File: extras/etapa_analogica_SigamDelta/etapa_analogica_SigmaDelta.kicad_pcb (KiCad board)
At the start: 2 copper layers, 63.5 x 78.8 mm, 19 parts, among them P1 CONN_02X10, P2 CONN_01X03, P3 CONN_02X10, P4 BNC

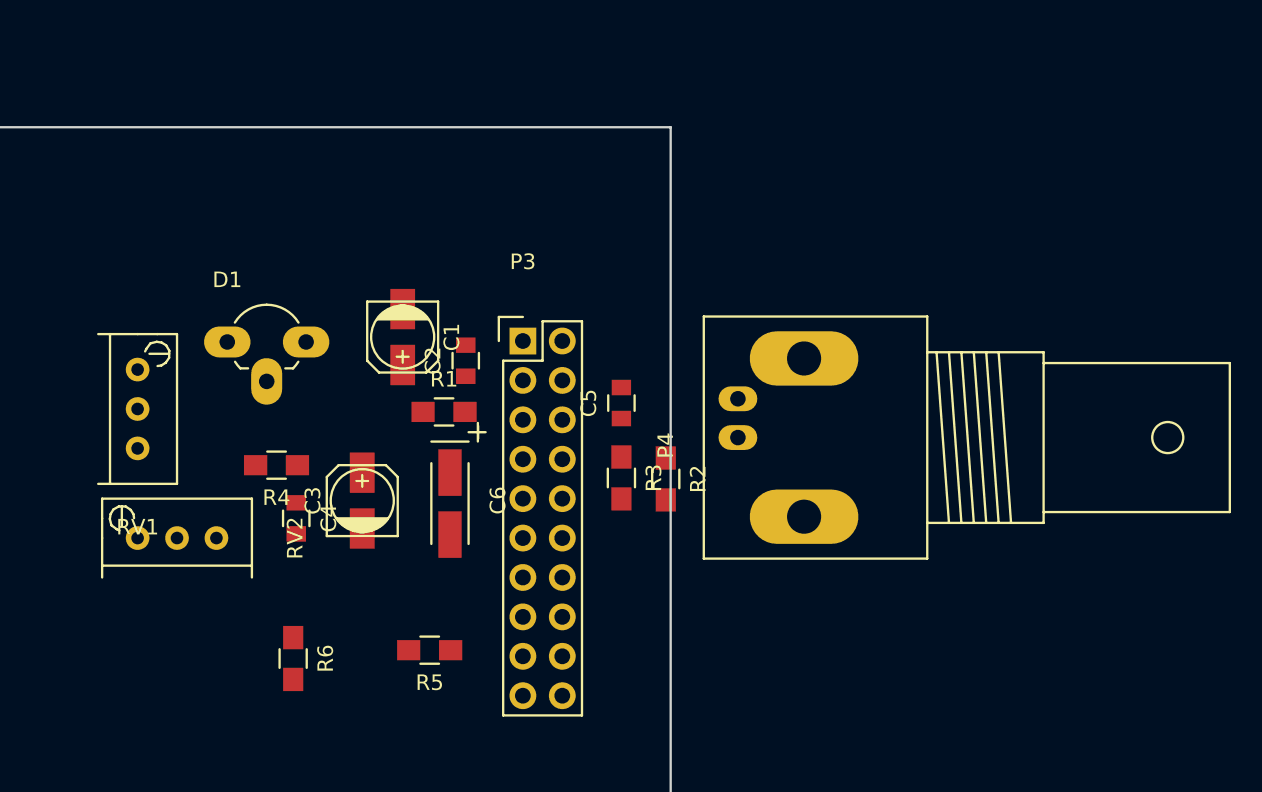
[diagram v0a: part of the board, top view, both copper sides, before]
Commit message: chasis bnc
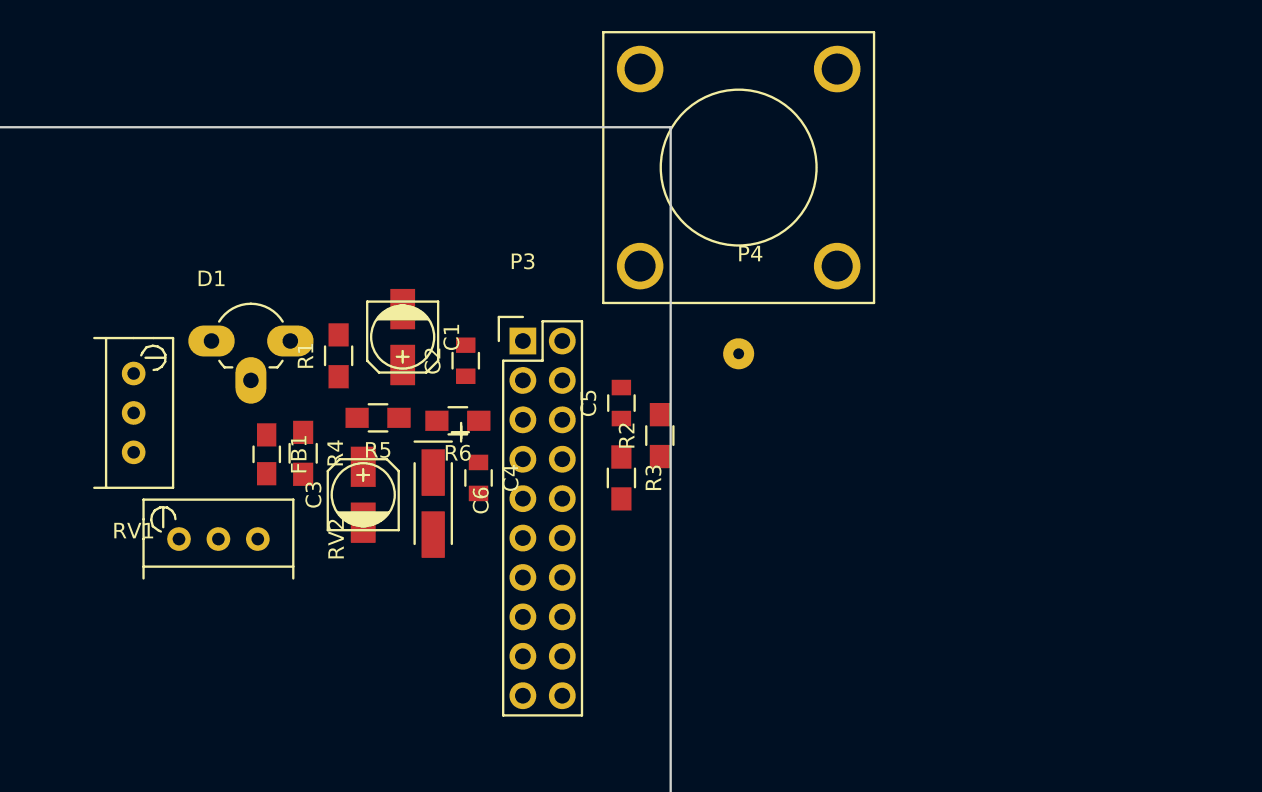
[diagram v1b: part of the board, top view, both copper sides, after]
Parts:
- added FB1: FILTER, Capacitors_SMD:C_0805_HandSoldering, F.Cu at (123.8, 76.9)
- P4: footprint Sockets_BNC:BNC_Socket_TYCO-AMP_LargePads -> chasis_bnc:chasis_bnc
- moved R6 18.6 mm to (136.1, 74.7), turned to 180 degrees
- moved P4 18.1 mm to (154.2, 58.4), turned to 0 degrees
- moved R5 15.3 mm to (131.0, 74.5)
- moved C4 12.0 mm to (137.5, 78.4)
- moved R1 7.70 mm to (128.5, 70.5), turned to 90 degrees
- moved R2 2.82 mm to (149.2, 75.7), turned to 90 degrees
- moved RV2 2.67 mm to (118.2, 82.4)
- moved R4 1.88 mm to (126.2, 76.8), turned to 270 degrees
- moved C6 1.08 mm to (134.6, 80.1)
- moved D1 1.02 mm to (120.3, 69.6)
- moved C3 0.39 mm to (130.0, 79.5)
- moved RV1 0.36 mm to (115.3, 71.7)
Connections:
- D1 pad 1: Net-(D1-Pad1) -> GND
- D1 pad 2: GND -> Net-(D1-Pad2)
- D1 pad 3: (no net) -> Net-(D1-Pad3)
- P1 pad 10: /Tx -> Net-(P1-Pad10)
- P1 pad 12: Net-(P1-Pad12) -> /Tx
- P1 pad 14: Net-(P1-Pad14) -> /Rx
- P1 pad 8: /Rx -> Net-(P1-Pad8)
- R1 pad 1: Net-(D1-Pad1) -> Net-(D1-Pad2)
- RV1 pad 1: Net-(D1-Pad1) -> Net-(D1-Pad2)
